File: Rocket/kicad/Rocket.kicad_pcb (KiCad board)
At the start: 2 copper layers, 143.2 x 107.6 mm, 29 parts, among them T1 Q_NPN_EBC, T2 Q_NPN_EBC, U1 NE555P, U2 BAT_HLD_SMD

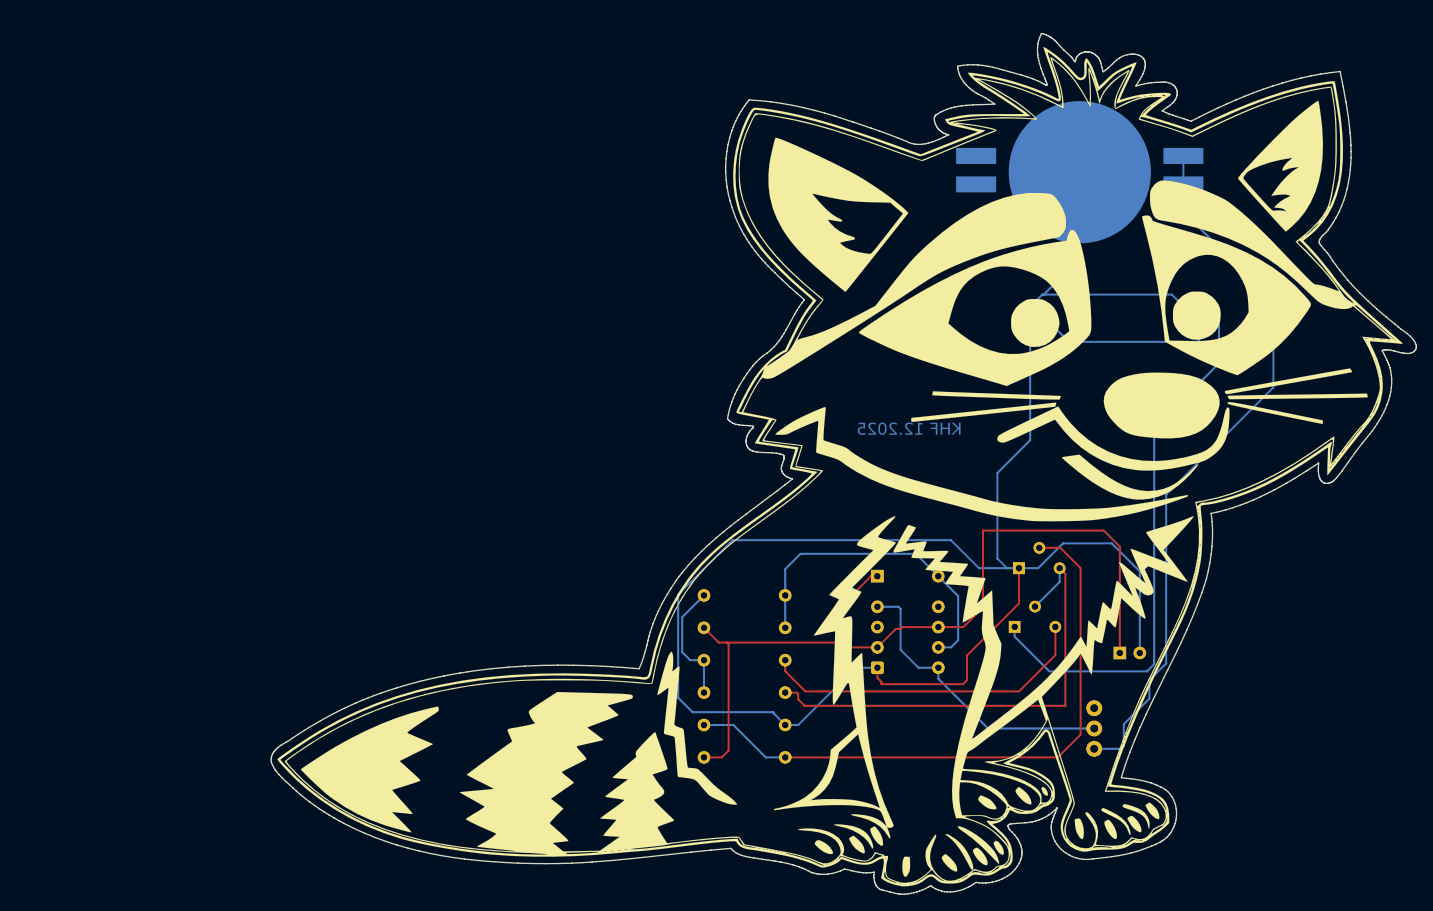
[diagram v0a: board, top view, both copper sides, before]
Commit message: V07122025
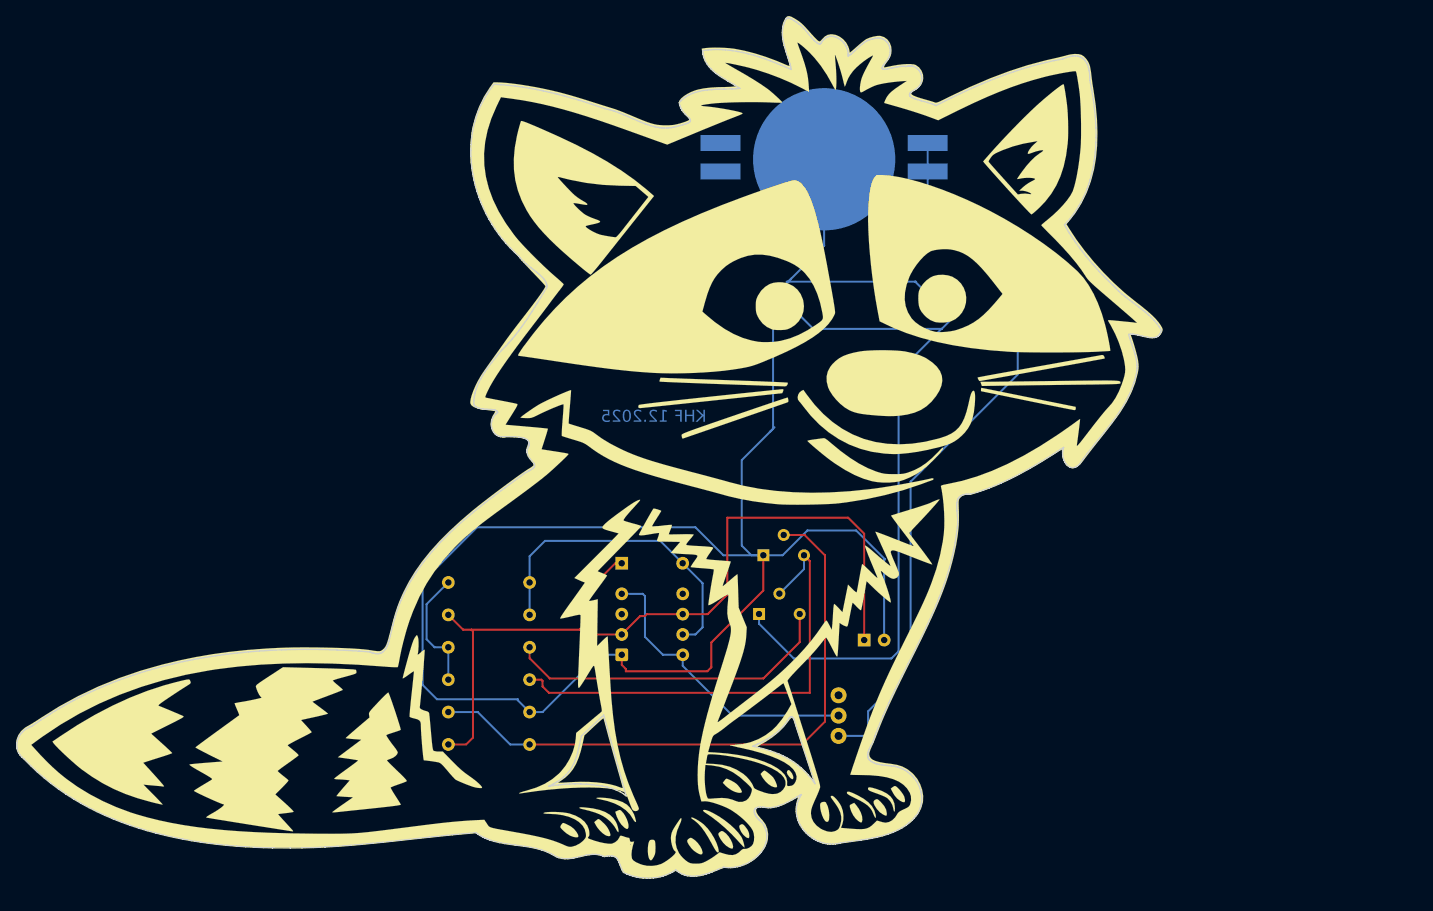
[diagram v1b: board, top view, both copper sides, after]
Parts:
- removed the G*** at (142.5, 100.8) (x7)
- removed the G*** at (142.7, 100.8) (x6)
- added G*** (x6): LOGO, LOGO, F.Cu at (110.7, 99.2)
- added G*** (x7): LOGO, LOGO, F.Cu at (110.8, 96.5)
- added G*** (x6): LOGO, LOGO, F.Cu at (110.5, 99.2)
- moved D1 32.2 mm to (135.4, 76.3)
- moved D2 32.0 mm to (155.3, 75.4)
- moved S1 32.0 mm to (143.5, 130.0)
- moved T1 32.0 mm to (134.1, 107.4)
- moved T2 32.0 mm to (133.6, 114.7)
- moved U1 32.0 mm to (116.4, 119.8)
- moved D3 32.0 mm to (116.4, 108.4)
- moved G*** 32.0 mm to (125.5, 99.0)
- moved R1off1 32.0 mm to (94.8, 110.8)
- moved R3 32.0 mm to (94.8, 131.0)
- moved R4 32.0 mm to (94.8, 127.0)
- moved R5 32.0 mm to (94.8, 122.9)
- moved R6 32.0 mm to (94.8, 118.9)
- moved R7 32.0 mm to (94.8, 114.8)
- moved 47uF 32.0 mm to (146.7, 118.0)
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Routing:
- net Net-(D1-A): track 91.5 -> 86.6 mm
- net Net-(D1-K): track 222.4 -> 226.1 mm
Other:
- board size 143.2 x 107.6 mm -> 143.1 x 107.5 mm
